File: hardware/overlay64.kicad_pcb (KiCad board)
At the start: 2 copper layers, 44.5 x 58.4 mm, 30 parts, among them IC1 ATMEGA1284-P, P1 USB, P2 INPUT, P3 CONTROL, P4 MAIN, P5 HOLE, P6 HOLE, P7 HOLE, P8 HOLE, P9 BYPASS, Q1 BC547B, U1 LM1881, Y1 20MHz

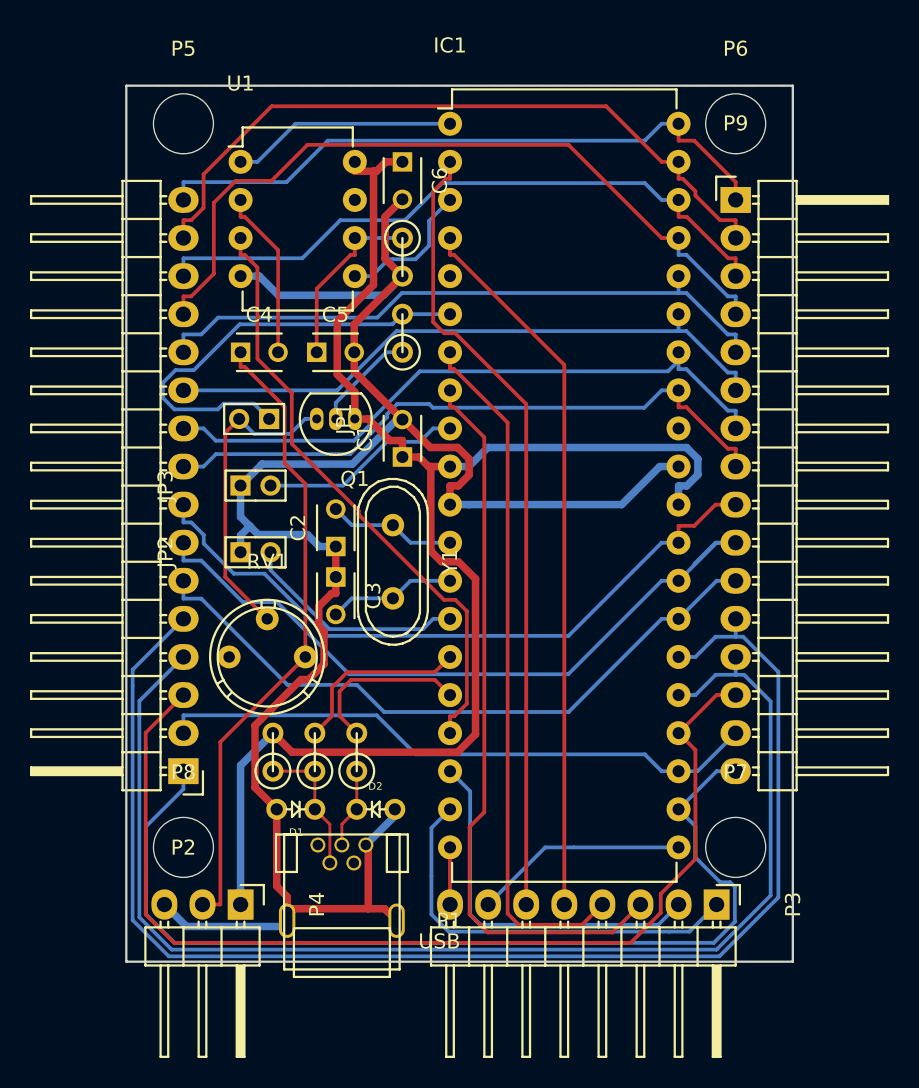
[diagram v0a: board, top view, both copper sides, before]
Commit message: Hardware: Prototype 2, rearranged, rerouted, added gerber files
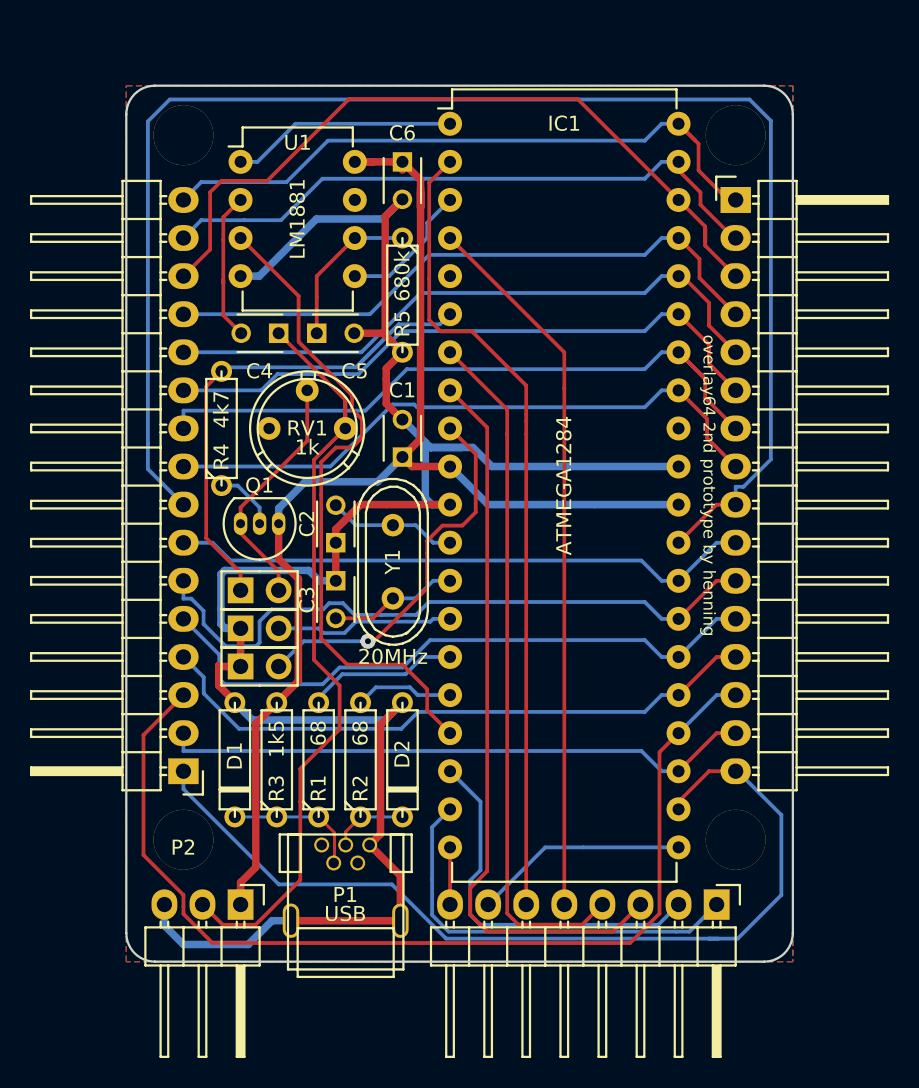
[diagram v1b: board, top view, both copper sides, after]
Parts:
- D1, D2: value 3.6V -> 3.6; footprint custom:Diode-2.5mm-Vertical -> custom:D3
- IC1: value ATMEGA1284-P -> ATMEGA1284
- JP1, JP2, JP3: footprint custom:Pin_Header_Straight_1x02_Pitch2.00mm -> custom:Pin_Header_Straight_1x02
- R1, R2, R3, R4, R5: footprint custom:R1 -> Discret:R3
- moved RV1 15.5 mm to (125.1, 83.8)
- moved R4 13.6 mm to (121.9, 83.8)
- moved JP3 12.1 mm to (123.2, 99.7)
- moved JP1 11.6 mm to (123.2, 94.6), turned to 90 degrees
- moved Q1 8.64 mm to (125.7, 90.2)
- moved D1 5.24 mm to (122.8, 105.9), turned to 90 degrees
- moved JP2 5.08 mm to (123.2, 97.2)
- moved D2 3.75 mm to (134.0, 105.9), turned to 90 degrees
- moved C4 2.84 mm to (125.7, 77.5), turned to 180 degrees
- moved R5 2.54 mm to (134.0, 74.9)
- moved C5 1.27 mm to (128.3, 77.5)
- moved P5 0.76 mm to (119.4, 64.3)
- moved P6 0.76 mm to (156.2, 64.3)
- moved R1 0.57 mm to (128.4, 105.9)
- moved R2 0.57 mm to (131.2, 105.9)
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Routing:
- net /IN8: track 45.8 -> 101.0 mm
- net /IN11: track 91.6 -> 42.3 mm
- net /IN12: track 84.6 -> 41.4 mm
- net VCC: track 98.3 -> 85.9 mm
- net /~RESET: track 13.5 -> 25.6 mm, vias 0 -> 1
- net /IN3: track 51.0 -> 41.8 mm
- net /IN9: track 48.1 -> 38.9 mm
- net /LUMA: track 42.3 -> 51.3 mm
- net /IN2: track 44.0 -> 50.6 mm
- net /MOSI: track 30.0 -> 36.3 mm
- net /IN1: track 47.6 -> 42.0 mm
- net Net-(IC1-Pad16): track 11.4 -> 6.61 mm
- net GND: track 132.7 -> 137.3 mm
- net /IN15: track 65.5 -> 61.8 mm
- net Net-(JP1-Pad2): track 20.9 -> 17.2 mm
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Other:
- outline, holes or cut-outs redrawn
- board text added: "overlay64 2nd prototype by henning"
